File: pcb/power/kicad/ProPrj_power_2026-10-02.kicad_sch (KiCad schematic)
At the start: 0 parts

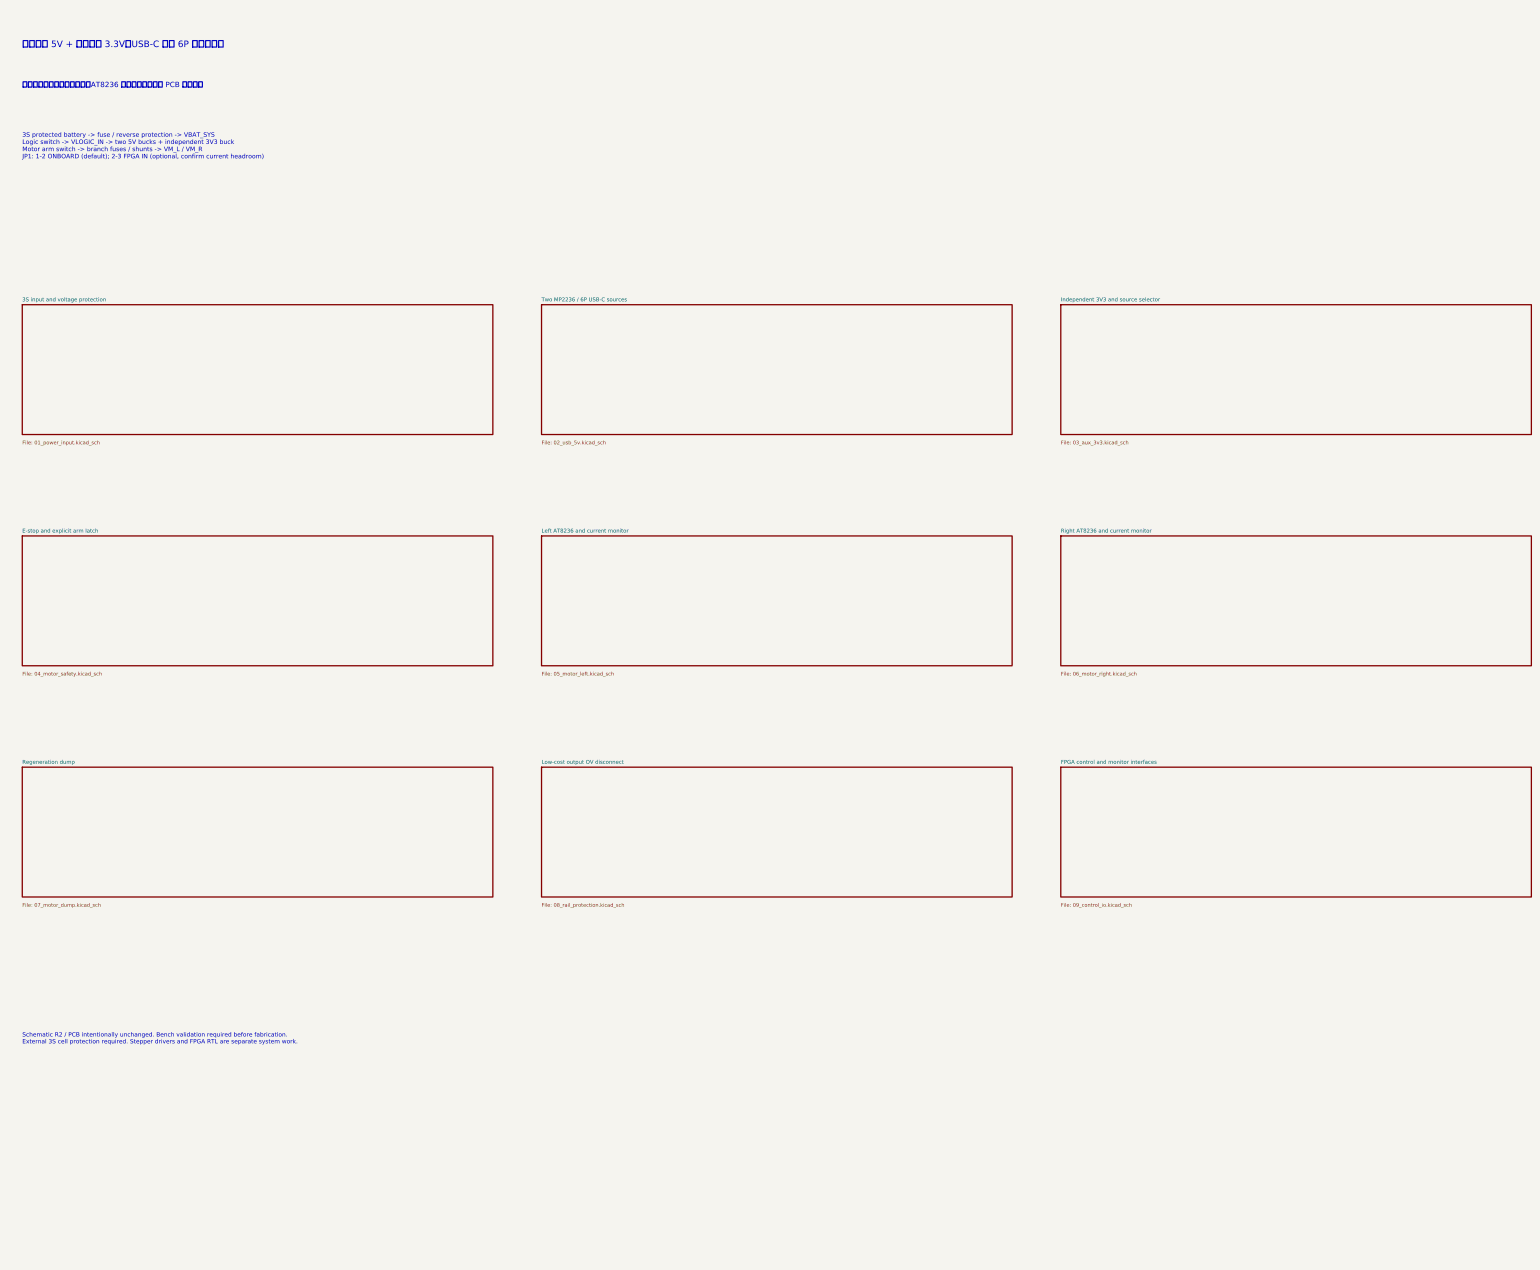
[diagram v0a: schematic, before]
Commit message: 10.3
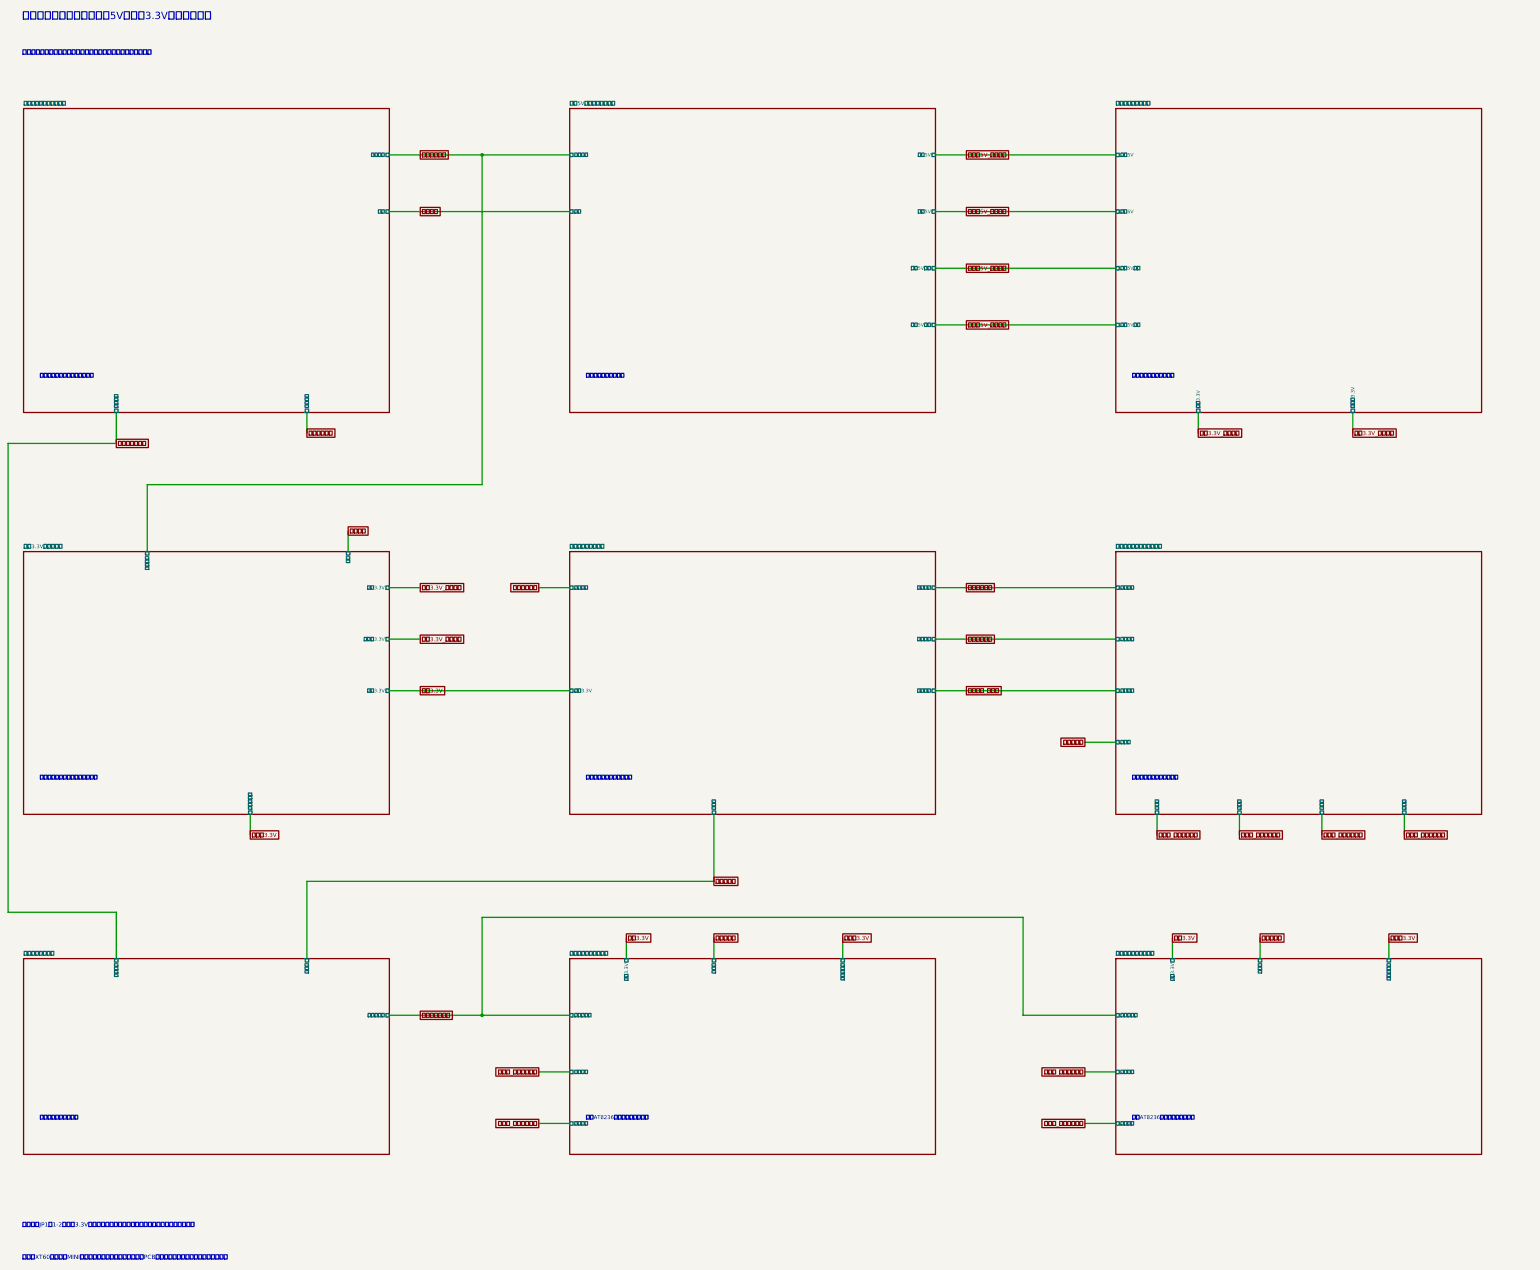
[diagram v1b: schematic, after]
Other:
- sheet 3S input and voltage protection renamed 三串电池输入与电压保护
- sheet E-stop and explicit arm latch renamed 急停与显式解锁锁存
- sheet FPGA control and monitor interfaces renamed 逻辑板控制与电源监测接口
- sheet Independent 3V3 and source selector renamed 独立3.3V与电源选择
- sheet Left AT8236 and current monitor renamed 左电机驱动与电流监测
- sheet Low-cost output OV disconnect renamed 低成本输出过压关断
- sheet Regeneration dump renamed 电机回生能量泄放
- sheet Right AT8236 and current monitor renamed 右电机驱动与电流监测
- sheet Two MP2236 / 6P USB-C sources renamed 两路5V降压与六针供电口
- sheet 三串电池输入与电压保护 ports: added 使能, 动力正常, 电池母线, 降压输入; removed none
- sheet 两路5V降压与六针供电口 ports: added 使能, 计算5V, 计算5V保护, 逻辑5V, 逻辑5V保护, 降压输入; removed none
- sheet 低成本输出过压关断 ports: added 保护后3.3V, 板载3.3V, 计算5V, 计算5V保护, 逻辑5V, 逻辑5V保护; removed none
- sheet 右电机驱动与电流监测 ports: added 传感器电源, 反转脉宽, 已解锁, 本板3.3V, 正转脉宽, 电机总电源; removed none
- sheet 左电机驱动与电流监测 ports: added 传感器电源, 反转脉宽, 已解锁, 本板3.3V, 正转脉宽, 电机总电源; removed none
- sheet 急停与显式解锁锁存 ports: added 动力正常, 外部故障, 已解锁, 本板3.3V, 解锁脉冲, 运行许可; removed none
- sheet 独立3.3V与电源选择 ports: added 传感器电源, 使能, 保护后3.3V, 本板3.3V, 板载3.3V, 降压输入; removed none
- sheet 电机回生能量泄放 ports: added 已解锁, 电机总电源, 电池母线; removed none
- sheet 逻辑板控制与电源监测接口 ports: added 右反转, 右正转, 外部故障, 左反转, 左正转, 已解锁, 解锁脉冲, 运行许可; removed none
- note added: "两路降压与六针供电口"
- note added: "动力总开关与回生泄放"
- note added: "右侧AT8236、编码器与电流监测"
- note added: "实线为实际层级网络连接；远距离控制、监测信号采用同名标签。"
- note added: "左侧AT8236、编码器与电流监测"
- note added: "急停、上电复位与解锁锁存"
- note added: "板载总保险、防反接与电压窗口"
- note added: "独立降压、跳帽选择与传感器滤波"
- note added: "电池经XT60接入板载MINI总保险；单体电芯保护仍须落实。PCB封装与网络已同步，布局布线待完成。"
- note added: "电源板功能连接总图：两路5V、独立3.3V与双电机驱动"
- note added: "输出过压与动力过流检测"
- note added: "逻辑板控制与电源监测接口"
- note added: "默认短接JP1的1-2：板载3.3V。只安装一个跳帽；电机故障恢复后须重新发解锁脉冲。"
- note removed: "3S protected battery -> fuse / reverse protection -> VBAT_SYS Logic switch -> VLOGIC_IN -> two 5V bucks + independent 3V3 buck Motor arm switch -> branch fuses / shunts -> VM_L / VM_R JP1: 1-2 ONBOARD (default); 2-3 FPGA IN (optional, confirm current headroom)"
- note removed: "Schematic R2 / PCB intentionally unchanged. Bench validation required before fabrication. External 3S cell protection required. Stepper drivers and FPGA RTL are separate system work."
- note removed: "两路独立 5V + 默认独立 3.3V；USB-C 使用 6P 供电插座。"
- note removed: "区内实线连接；跨模块标签。AT8236 使用两排排母；原 PCB 不更新。"
- company: EdgeMind Robot -> EdgeMind机器人
- title: EdgeMind Robot power / 2x5V + independent 3V3 -> 机器人电源板 / 两路5V与独立3.3V
